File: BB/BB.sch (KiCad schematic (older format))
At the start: 234 parts, among them SW0 SW_Push, U1 AT90USB1286-AU, Y0 16Mhz

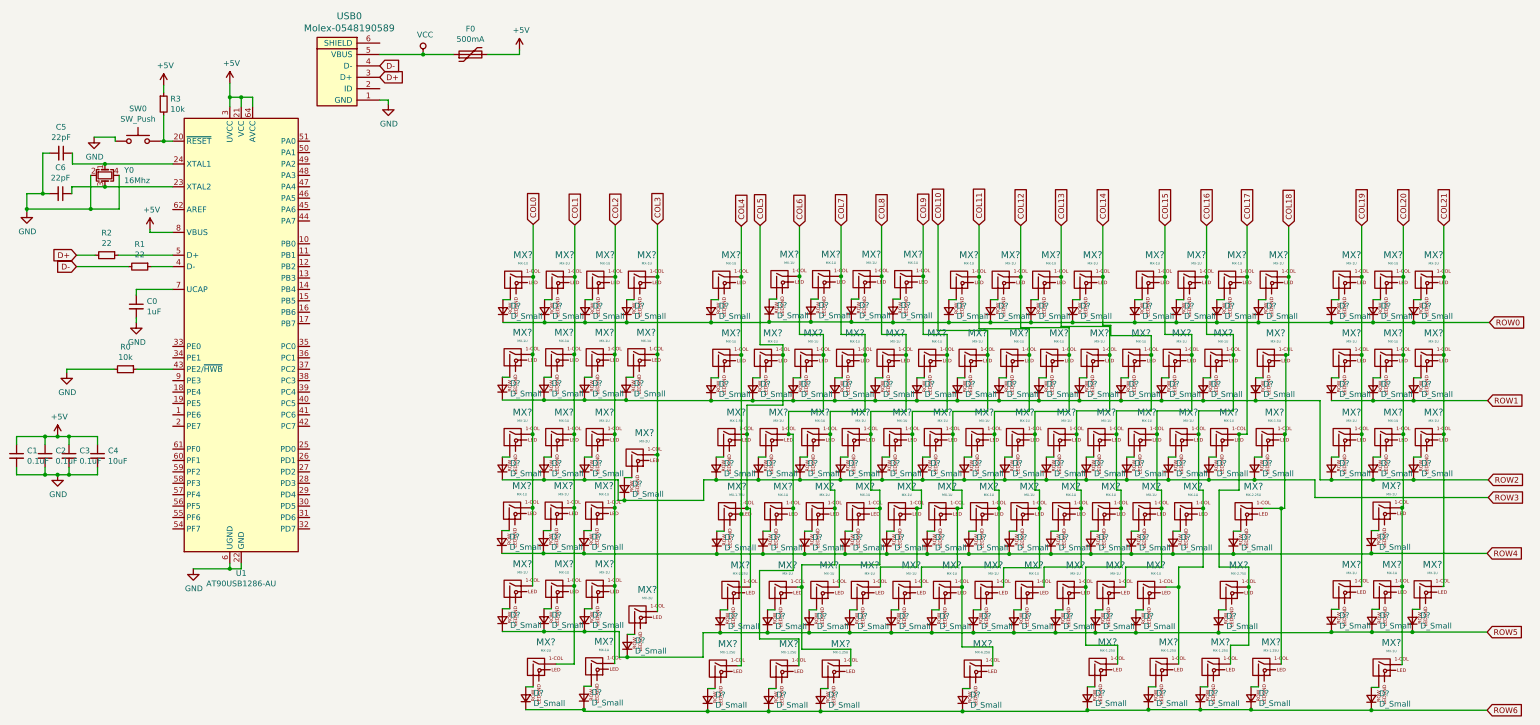
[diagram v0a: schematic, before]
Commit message: Finished Schematic
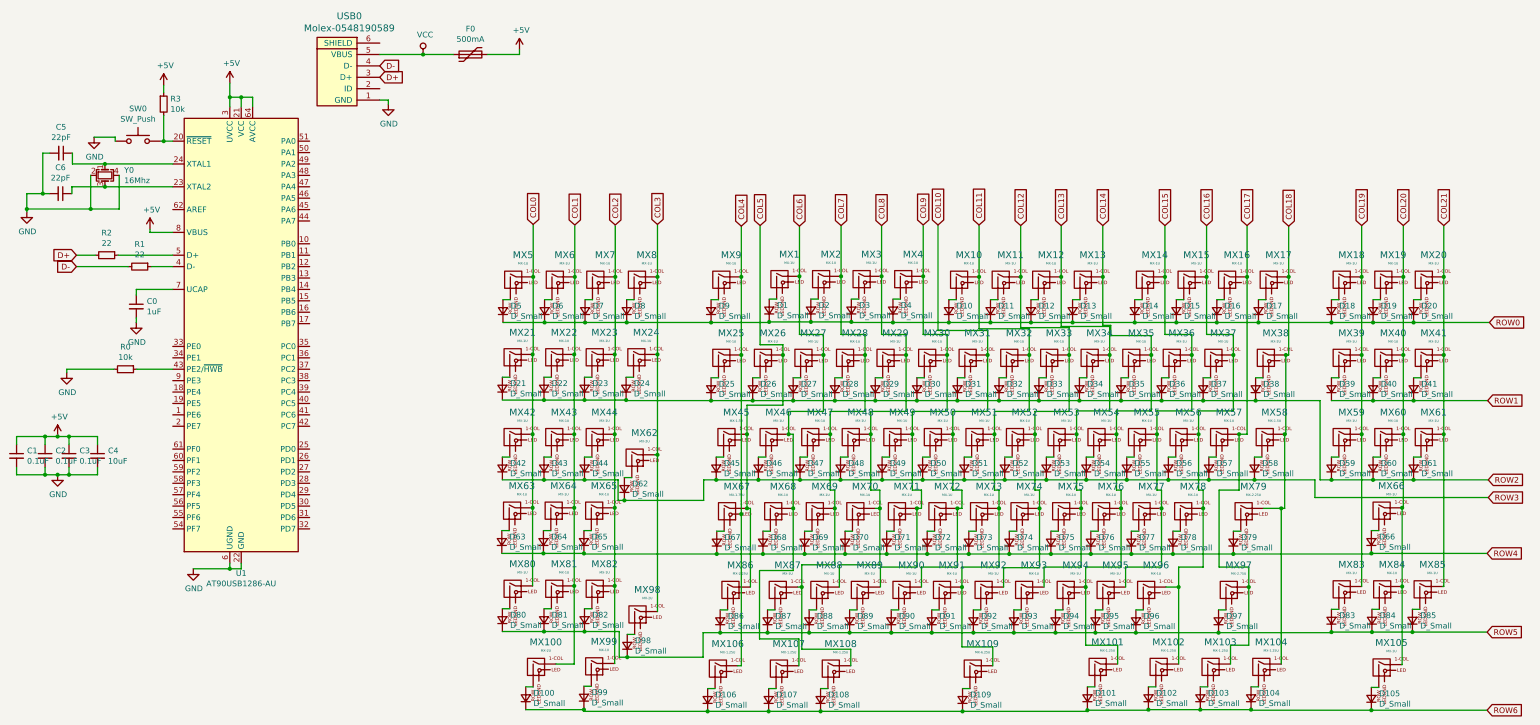
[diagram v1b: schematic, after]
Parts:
- C0, C1, C2, C3, C4, C5, C6: footprint (none) -> Capacitor_SMD:C_0805_2012Metric
- D1, D10, D100, D101, D102, D103, D104, D105, D106, D107, D108, D109, D11, D12, D13, D14, D15, D16, D17, D18, D19, D2, D20, D21, D22, D23, D24, D25, D26, D27, D28, D29, D3, D30, D31, D32, D33, D34, D35, D36, D37, D38, D39, D4, D40, D41, D42, D43, D44, D45, D46, D47, D48, D49, D5, D50, D51, D52, D53, D54, D55, D56, D57, D58, D59, D6, D60, D61, D62, D63, D64, D65, D66, D67, D68, D69, D7, D70, D71, D72, D73, D74, D75, D76, D77, D78, D79, D8, D80, D81, D82, D83, D84, D85, D86, D87, D88, D89, D9, D90, D91, D92, D93, D94, D95, D96, D97, D98, D99: renamed from D?; footprint (none) -> Diode_SMD:D_SOD-123
- F0: footprint (none) -> Fuse:Fuse_1206_3216Metric
- MX1, MX10, MX105, MX11, MX12, MX13, MX14, MX15, MX16, MX17, MX18, MX19, MX2, MX20, MX21, MX22, MX23, MX24, MX25, MX26, MX27, MX28, MX29, MX3, MX30, MX31, MX32, MX33, MX34, MX35, MX36, MX37, MX38, MX39, MX4, MX40, MX41, MX42, MX43, MX44, MX46, MX47, MX48, MX49, MX5, MX50, MX51, MX52, MX53, MX54, MX55, MX56, MX57, MX59, MX6, MX60, MX61, MX62, MX63, MX64, MX65, MX66, MX68, MX69, MX7, MX70, MX71, MX72, MX73, MX74, MX75, MX76, MX77, MX78, MX8, MX80, MX81, MX82, MX83, MX84, MX85, MX87, MX88, MX89, MX9, MX90, MX91, MX92, MX93, MX94, MX95, MX96, MX99: renamed from MX?; footprint (none) -> MX_Alps_Hybrid:MX-1U
- MX100, MX98: renamed from MX?; footprint (none) -> MX_Alps_Hybrid:MX-2U
- MX101, MX102, MX103, MX104, MX106, MX107, MX108: renamed from MX?; footprint (none) -> MX_Alps_Hybrid:MX-1.25U
- MX109: renamed from MX?; footprint (none) -> MX_Alps_Hybrid:MX-6.25U
- MX45, MX58: renamed from MX?; footprint (none) -> MX_Alps_Hybrid:MX-1.5U
- MX67: renamed from MX?; footprint (none) -> MX_Alps_Hybrid:MX-1.75U
- MX79, MX86: renamed from MX?; footprint (none) -> MX_Alps_Hybrid:MX-2.25U
- MX97: renamed from MX?; footprint (none) -> MX_Alps_Hybrid:MX-2.75U
- R0, R1, R2, R3: footprint (none) -> Resistor_SMD:R_0805_2012Metric
- SW0: footprint (none) -> random-keyboard-parts:SKQG-1155865
- USB0: footprint (none) -> random-keyboard-parts:Molex-0548190589
- Y0: footprint (none) -> Crystal:Crystal_SMD_3225-4Pin_3.2x2.5mm
